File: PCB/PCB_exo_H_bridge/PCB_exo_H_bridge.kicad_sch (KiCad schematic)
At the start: 8 parts, among them J101 Conn_01x03, J102 Conn_01x02

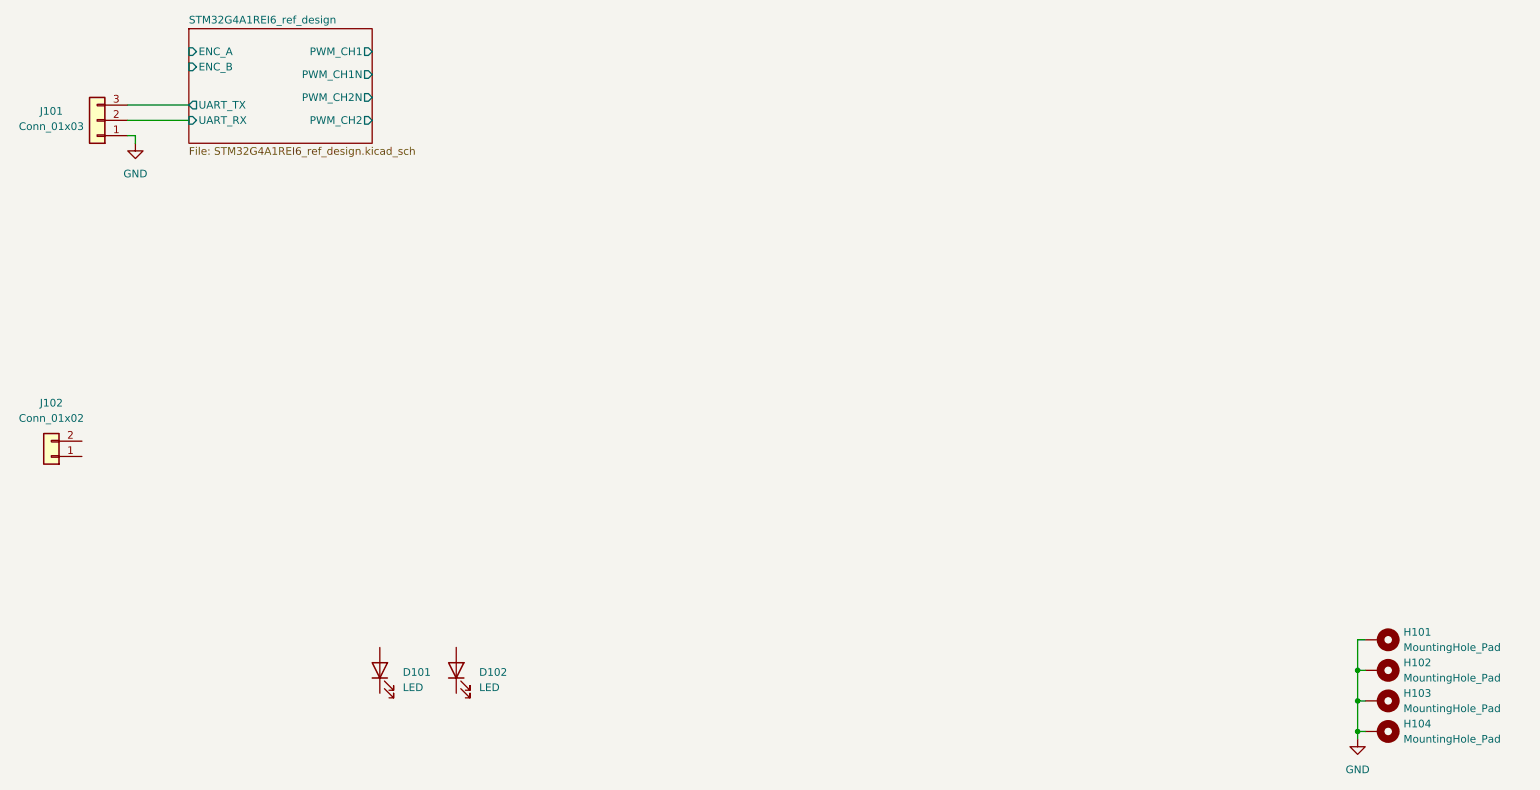
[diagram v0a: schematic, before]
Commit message: exo done
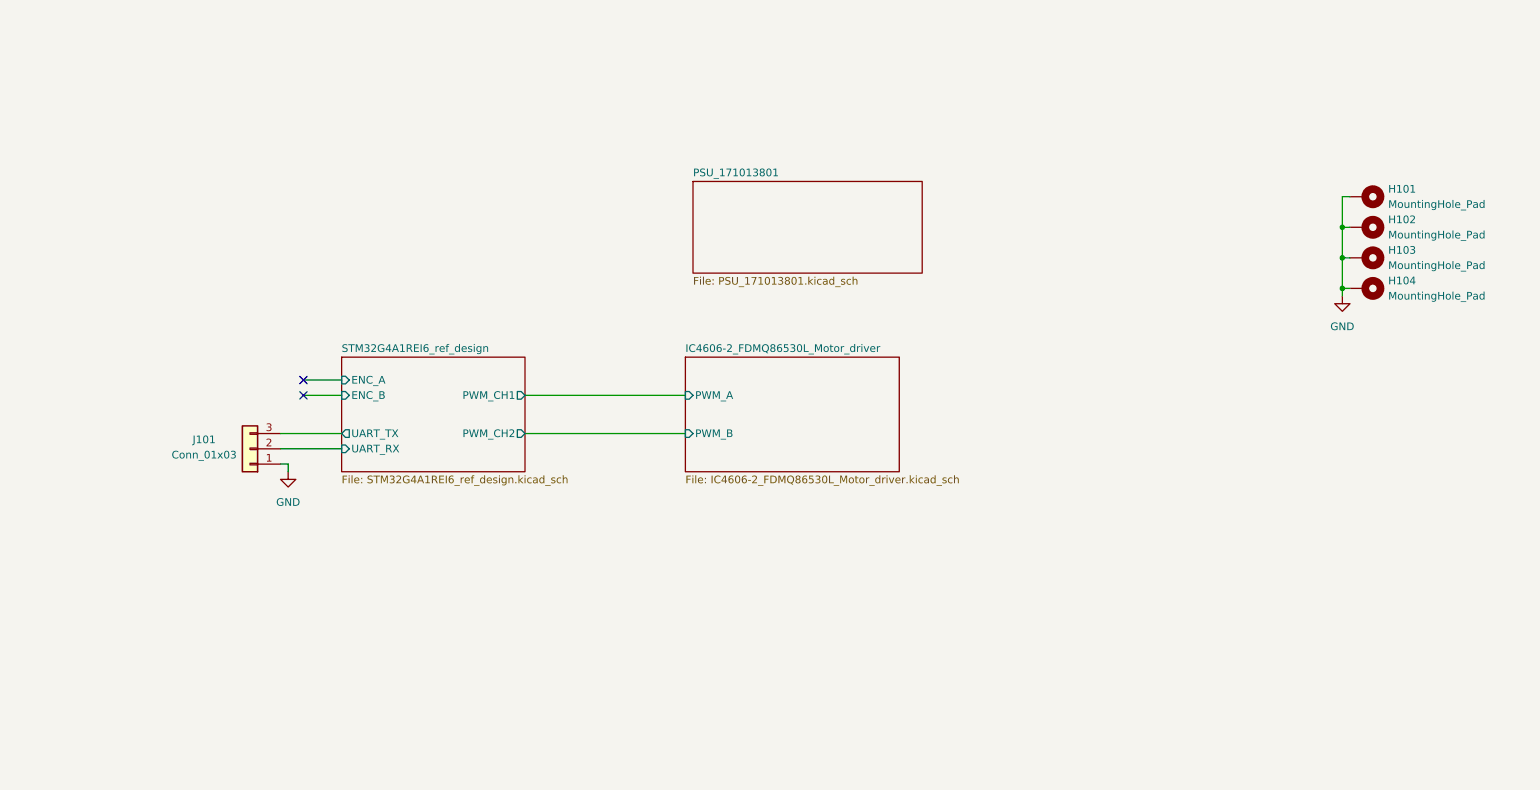
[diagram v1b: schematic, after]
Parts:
- removed D101, D102: LED, symbol Device:LED
- removed J102: Conn_01x02, symbol Connector_Generic:Conn_01x02
- H101, H102, H103, H104: footprint (none) -> MountingHole:MountingHole_2.7mm_M2.5_Pad_Via
- J101: footprint (none) -> Connector_JST:JST_EH_B3B-EH-A_1x03_P2.50mm_Vertical
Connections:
- no-connect marks 0 -> 2
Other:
- added sheet IC4606-2_FDMQ86530L_Motor_driver (IC4606-2_FDMQ86530L_Motor_driver.kicad_sch)
- added sheet PSU_171013801 (PSU_171013801.kicad_sch)
- sheet STM32G4A1REI6_ref_design ports: added none; removed PWM_CH1N, PWM_CH2N
- moved on the sheet: H101, H102, H103, H104, J101
